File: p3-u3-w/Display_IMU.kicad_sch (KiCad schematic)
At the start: 1 part, among them J2 SWD_pin

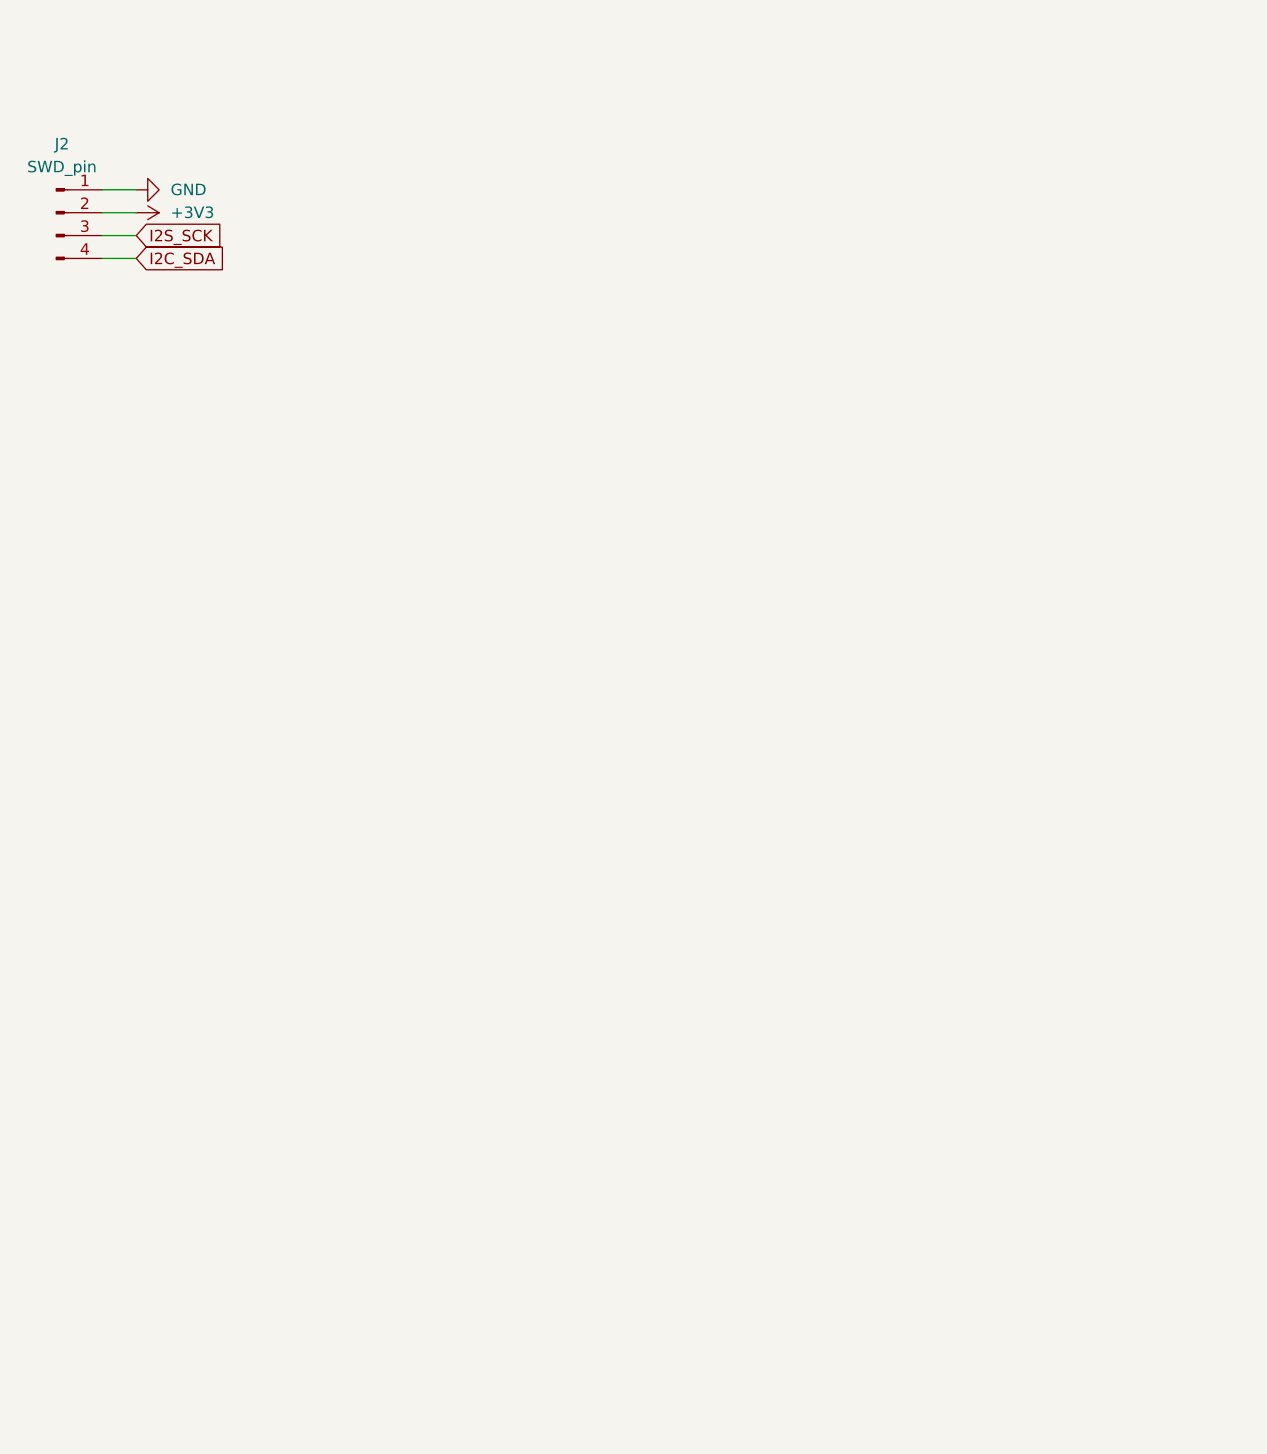
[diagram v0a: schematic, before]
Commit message: added in power side and mostly finished schematics :)
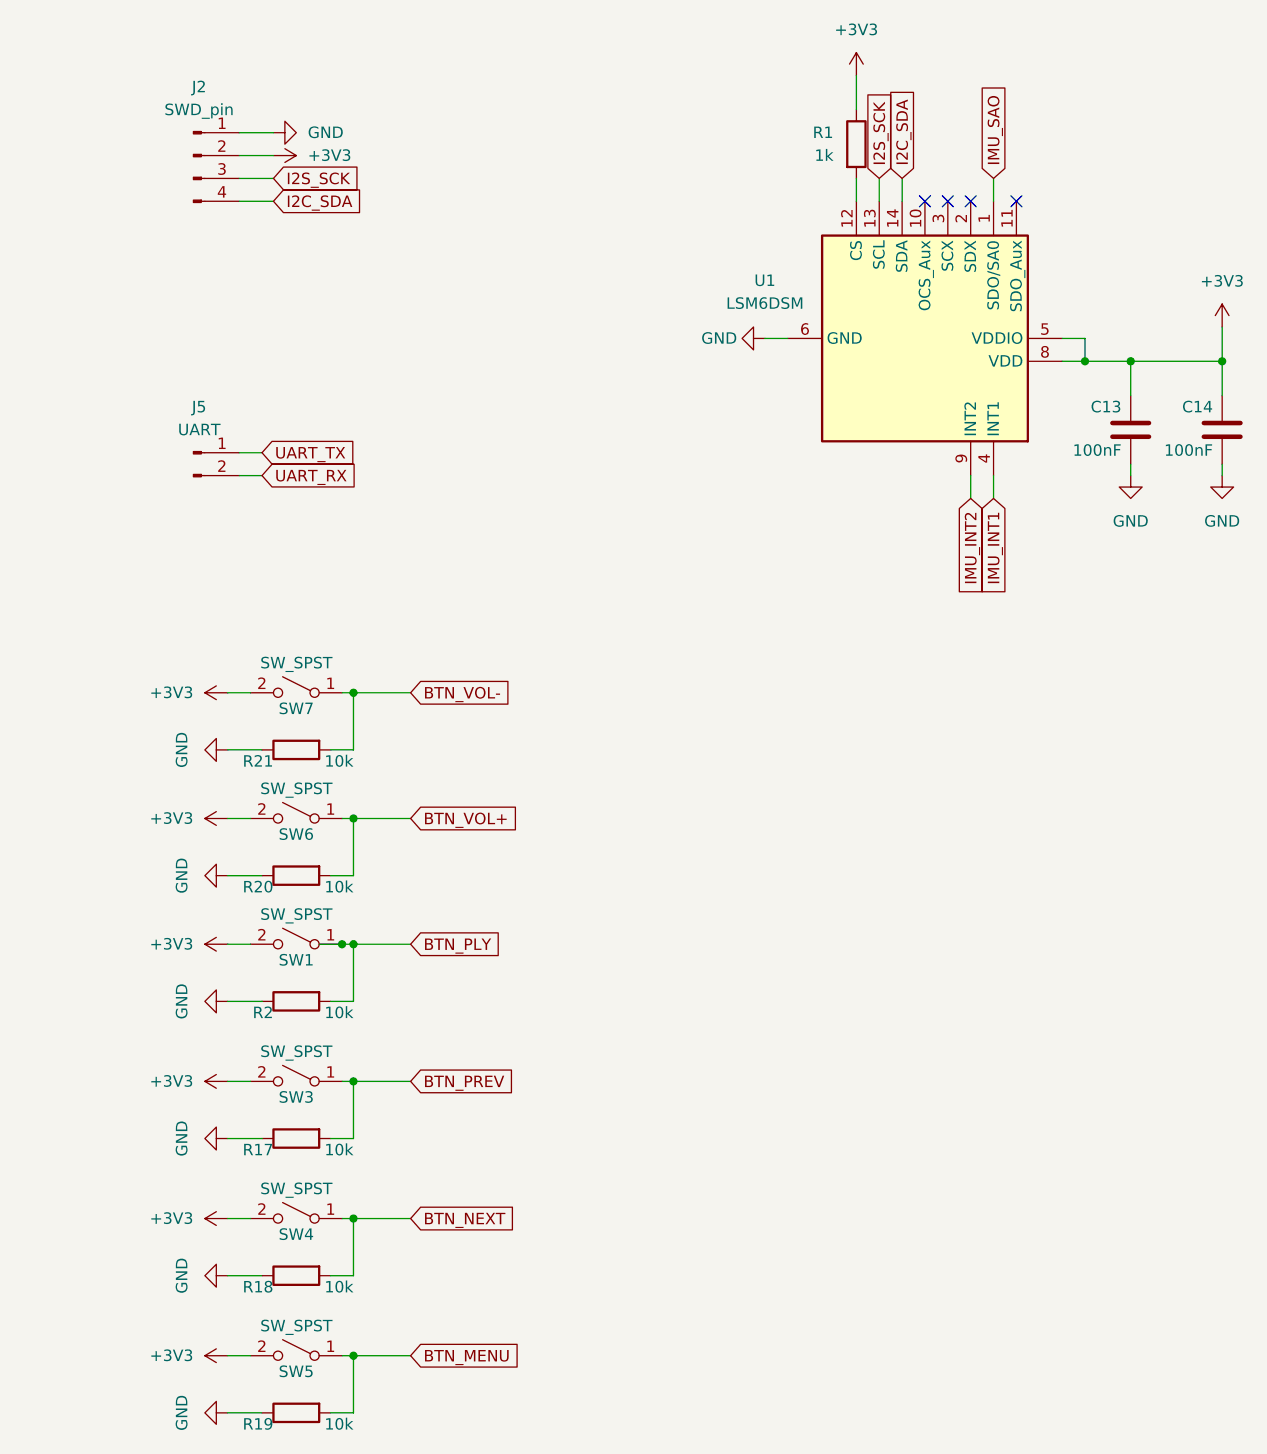
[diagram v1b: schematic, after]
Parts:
- added C13, C14: 100nF, symbol Device:C
- added J5: UART, symbol Connector:Conn_01x02_Pin
- added R1: 1k, symbol Device:R
- added R17, R18, R19, R2, R20, R21: 10k, symbol Device:R
- added SW1, SW3, SW4, SW5, SW6, SW7: SW_SPST, symbol Switch:SW_SPST
- added U1: LSM6DSM, Package_LGA:LGA-14_3x2.5mm_P0.5mm_LayoutBorder3x4y, symbol Sensor_Motion:LSM6DSM
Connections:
- net +3V3: now also C13.2, C14.2, R1.1, SW1.2 (B), SW3.2 (B), SW4.2 (B), SW5.2 (B), SW6.2 (B), SW7.2 (B), U1.5 (VDDIO), U1.8 (VDD)
- net GND: now also C13.1, C14.1, R17.1, R18.1, R19.1, R2.1, R20.1, R21.1, U1.6 (GND), U1.7 (GND)
- net I2C_SDA: now also U1.14 (SDA)
- net I2S_SCK: now also U1.13 (SCL)
- new net: R1.2, U1.12 (CS)
- new net BTN_MENU: R19.2, SW5.1 (A)
- new net BTN_NEXT: R18.2, SW4.1 (A)
- new net BTN_PLY: R2.2, SW1.1 (A)
- new net BTN_PREV: R17.2, SW3.1 (A)
- new net BTN_VOL+: R20.2, SW6.1 (A)
- new net BTN_VOL-: R21.2, SW7.1 (A)
- new net IMU_INT1: U1.4 (INT1)
- new net IMU_INT2: U1.9 (INT2)
- new net IMU_SAO: U1.1 (SDO/SA0)
- new net UART_RX: J5.2 (Pin_2)
- new net UART_TX: J5.1 (Pin_1)
- no-connect marks 0 -> 4
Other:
- moved on the sheet: J2
